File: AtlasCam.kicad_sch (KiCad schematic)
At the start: 37 parts, among them J1 SD_Micro_TFPUSH, J2 USB_C_16Pin_C167321, Q1 JTD6206-28, Q2 JTD6206-12, U1 ESP32-S3-WROOM-1(N8R8), U2 LDO_3V3_2A_AIC1221-33GY3TR, U3 05A20L24P

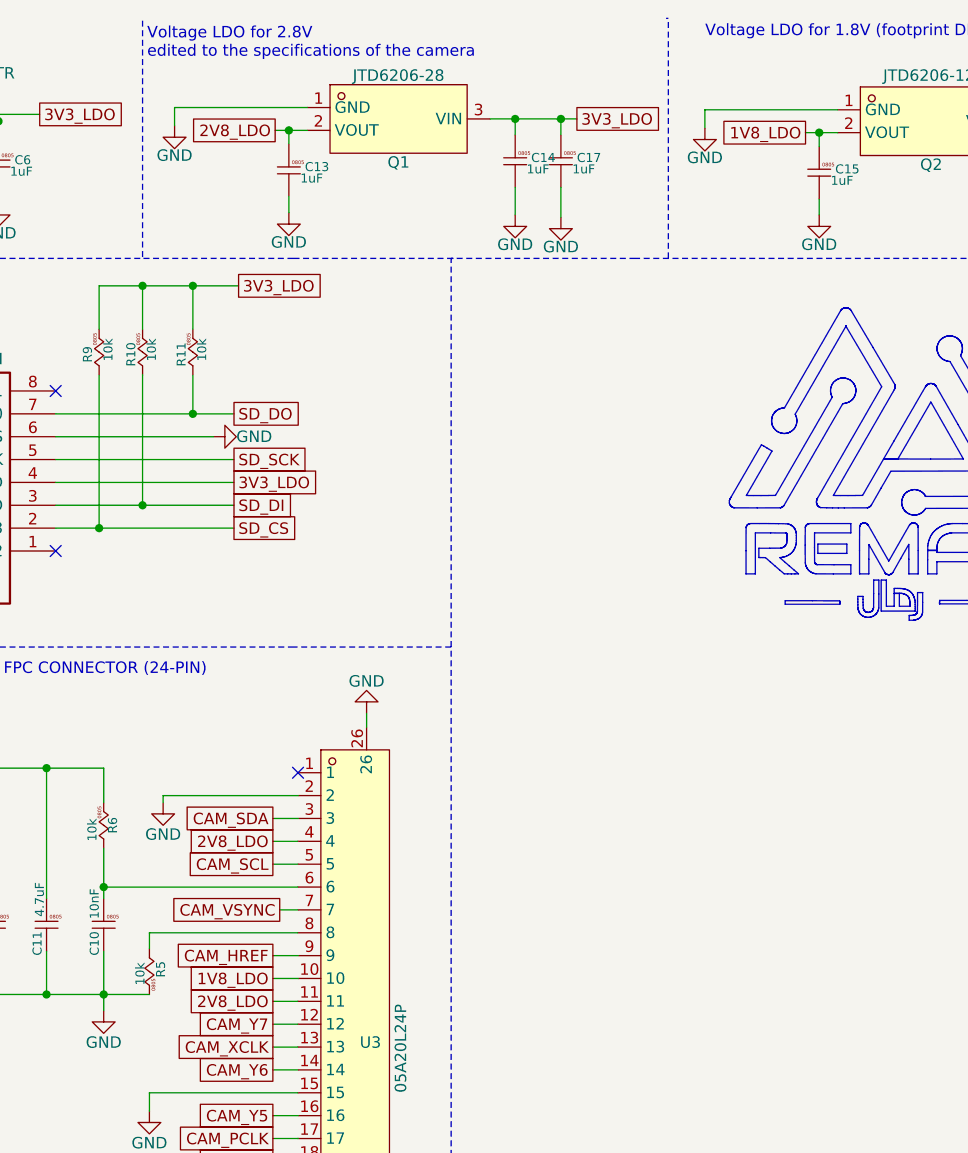
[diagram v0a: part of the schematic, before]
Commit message: Final Updates: pulled D-/D+ closer, moved SD Slot to edge, Verified design
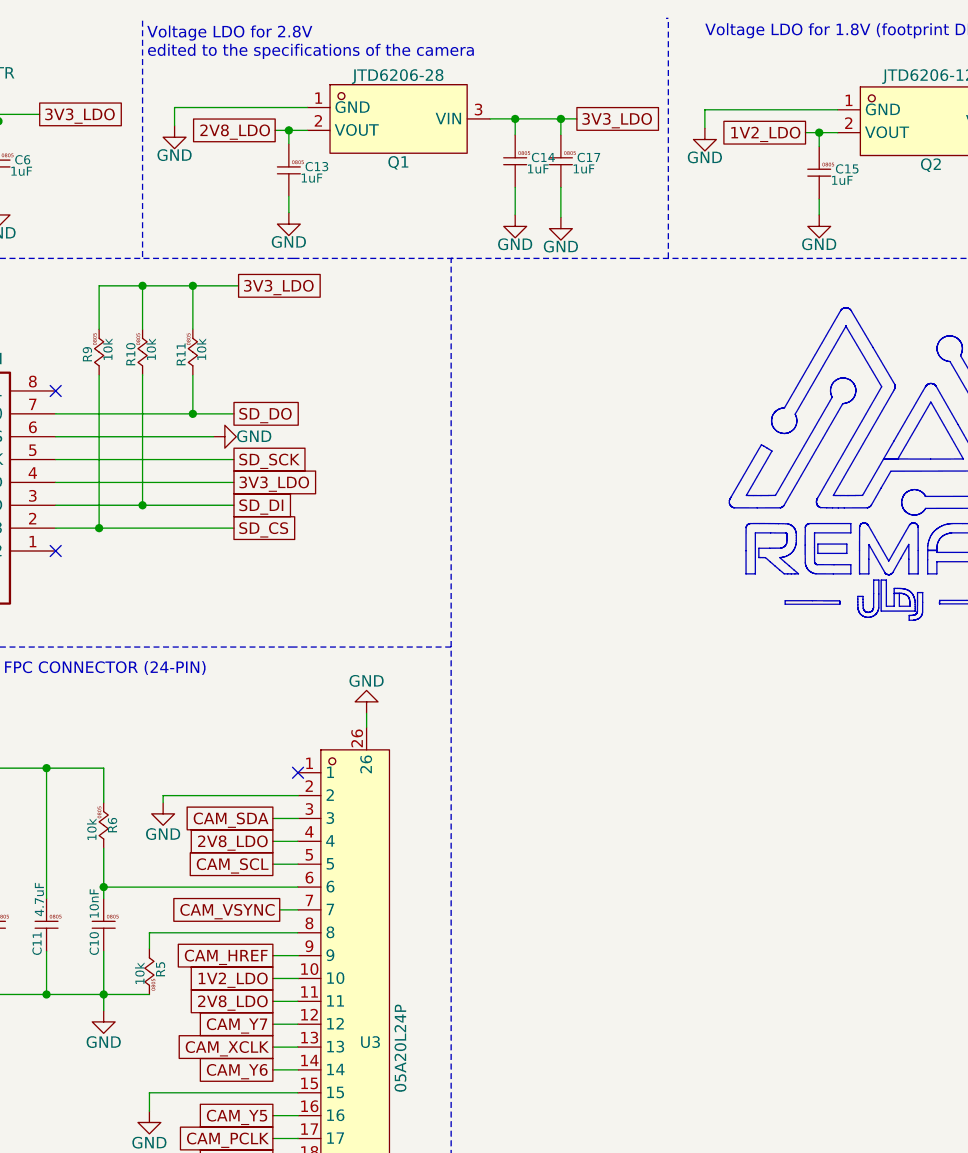
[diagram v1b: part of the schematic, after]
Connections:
- net 1V8_LDO renamed 1V2_LDO
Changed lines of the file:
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@@
 		)
 	)
-	(global_label "1V8_LDO"
+	(global_label "1V2_LDO"
 		(shape passive)
 		(at 211.328 24.638 180)
@@
 		)
 	)
-	(global_label "1V8_LDO"
+	(global_label "1V2_LDO"
 		(shape passive)
 		(at 152.146 118.618 180)
